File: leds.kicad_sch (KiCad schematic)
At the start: 64 parts

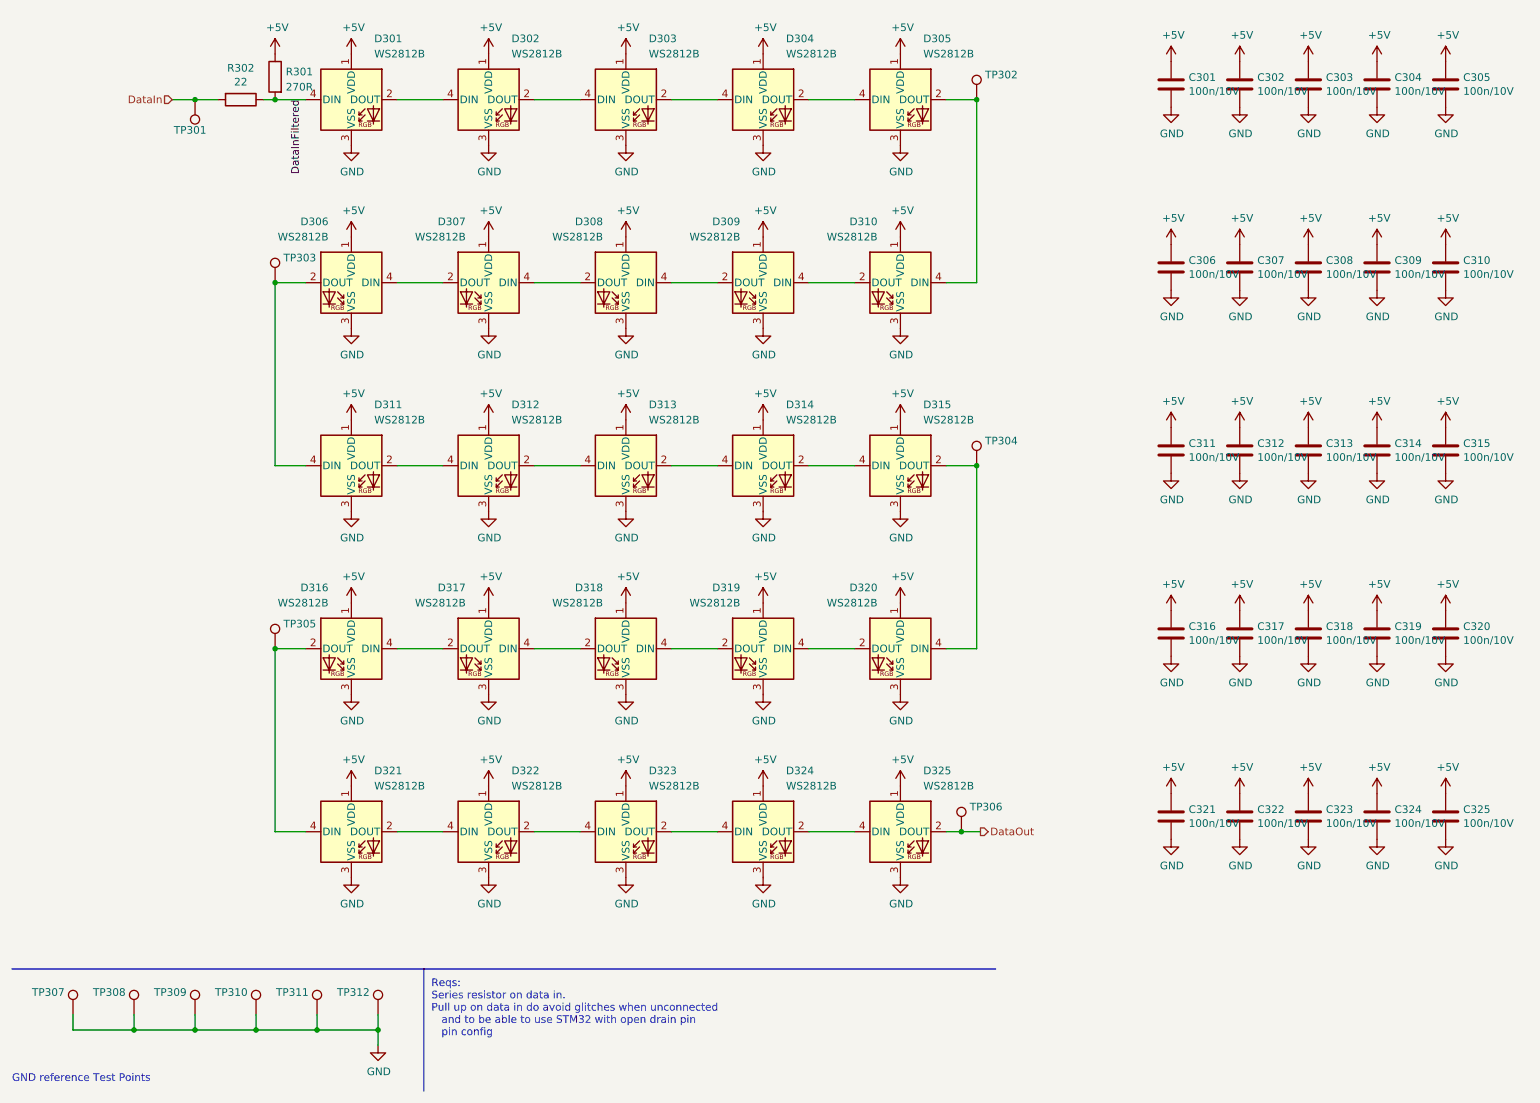
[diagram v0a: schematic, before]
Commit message: Final fixes before production
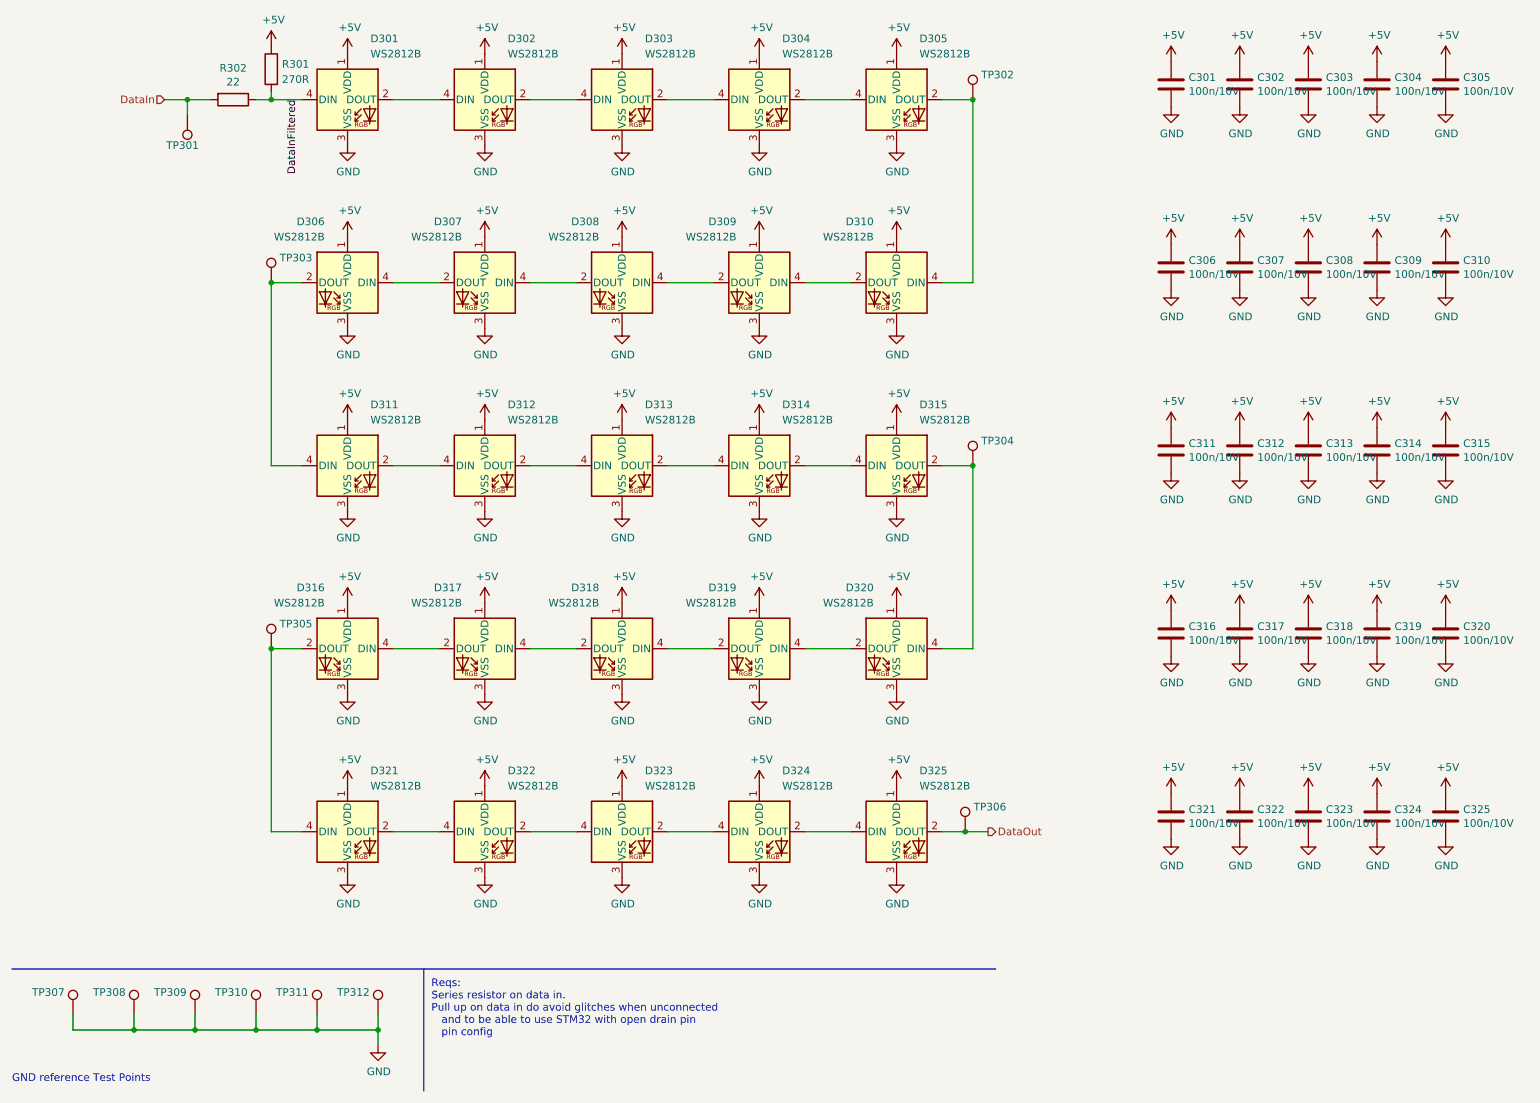
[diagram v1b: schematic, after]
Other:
- moved on the sheet: D301, D302, D303, D304, D305, D306, D307, D308, D309, D310, D311, D312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
